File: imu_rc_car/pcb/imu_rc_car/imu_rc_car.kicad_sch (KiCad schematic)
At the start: 27 parts, among them J1 Encoder FS, J10 Prox Sensor RS, J11 Prox Sensor LS, J12 Prox Sensor BS, J2 Encoder BS, J7 Left Terminal, J8 Right Terminal, J9 Prox Sensor FS, Q5 IRLML6344TRPBF, Q6 DMP3160L-7, U1 ESP32-S3-DevKitC, U2 TB6612FNG, U3 AP2112K-3.3, U4 TB6612FNG

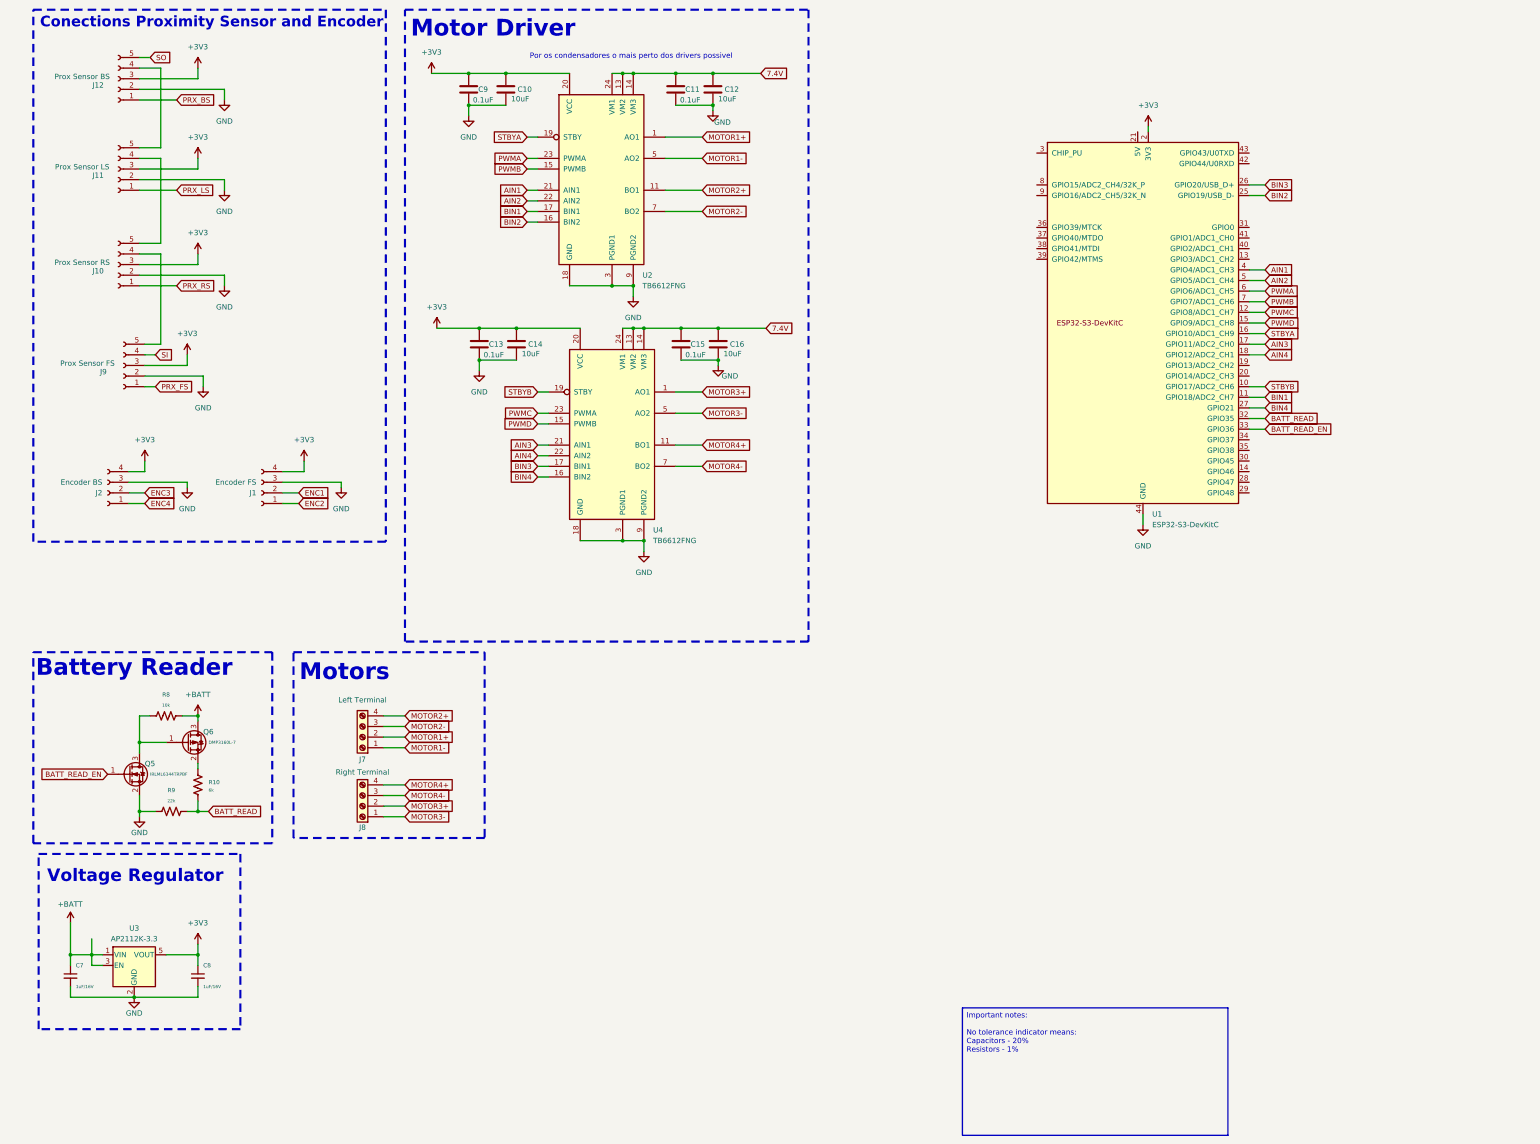
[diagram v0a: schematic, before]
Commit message: commit #27
revision for hand unit complete (board is ready)
board for proximity sensors in series
minor revision in encoder board
progressing work in car board
added essential libraries support for 3D components
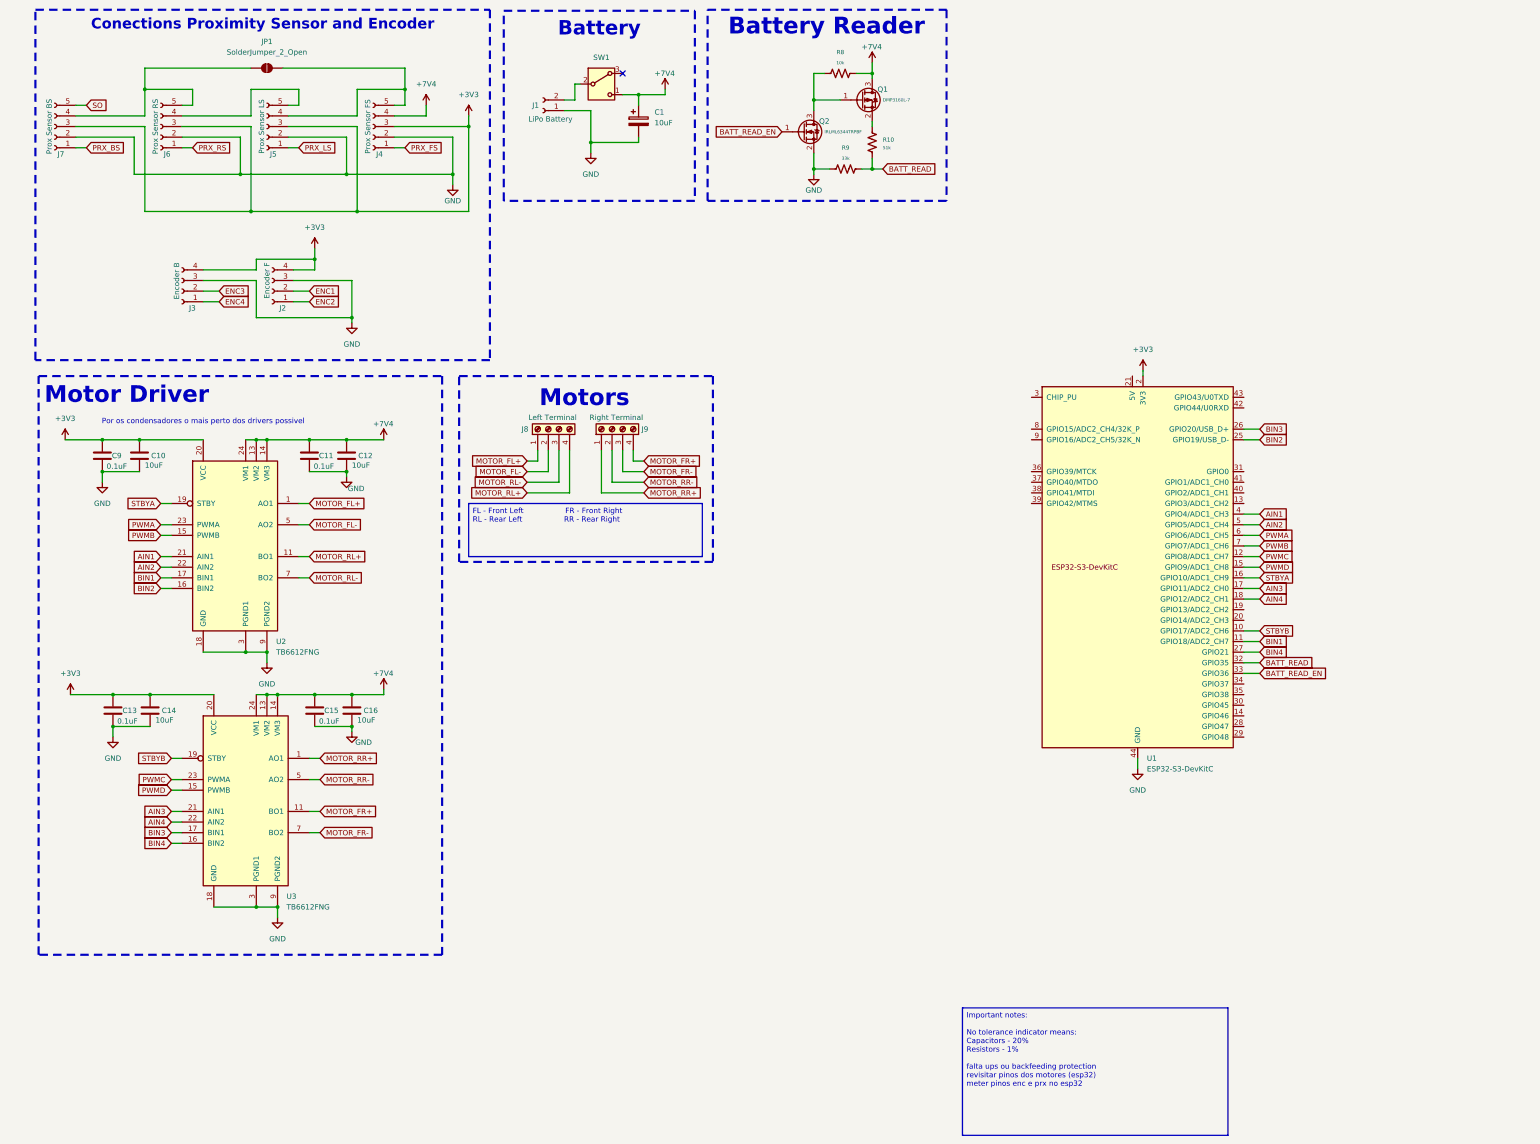
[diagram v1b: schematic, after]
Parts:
- removed C7, C8: 1uF/16V, Capacitor_SMD:C_0805_2012Metric, symbol Device:C_Small
- removed J10: Prox Sensor RS, Connector_JST:JST_PH_S5B-PH-K_1x05_P2.00mm_Horizontal, symbol Connector:Conn_01x05_Socket
- removed J11: Prox Sensor LS, Connector_JST:JST_PH_S5B-PH-K_1x05_P2.00mm_Horizontal, symbol Connector:Conn_01x05_Socket
- removed J12: Prox Sensor BS, Connector_JST:JST_PH_S5B-PH-K_1x05_P2.00mm_Horizontal, symbol Connector:Conn_01x05_Socket
- removed J2: Encoder BS, Connector_JST:JST_PH_S4B-PH-K_1x04_P2.00mm_Horizontal, symbol Connector:Conn_01x04_Socket
- removed U3: AP2112K-3.3, Package_TO_SOT_SMD:SOT-23-5, symbol Regulator_Linear:AP2112K-3.3
- added C1: 10uF, Capacitor_SMD:CP_Elec_5x5.7, symbol Device:C_Polarized
- added J1: LiPo Battery, IMURCLibrary:AMASS_XT60IPW-M_1x03_P7.20mm_Horizontal, symbol Connector:Conn_01x02_Socket
- added J3: Encoder B, IMURCLibrary:JST_PH_S4B-PH-SM4-TB_1x04-1MP_P2.00mm_Horizontal, symbol Connector:Conn_01x04_Socket
- added J5: Prox Sensor LS, IMURCLibrary:JST_PH_S5B-PH-SM4-TB_1x05-1MP_P2.00mm_Horizontal, symbol Connector:Conn_01x05_Socket
- added J6: Prox Sensor RS, IMURCLibrary:JST_PH_S5B-PH-SM4-TB_1x05-1MP_P2.00mm_Horizontal, symbol Connector:Conn_01x05_Socket
- added J7: Prox Sensor BS, IMURCLibrary:JST_PH_S5B-PH-SM4-TB_1x05-1MP_P2.00mm_Horizontal, symbol Connector:Conn_01x05_Socket
- added JP1: SolderJumper_2_Open, Jumper:SolderJumper-2_P1.3mm_Open_RoundedPad1.0x1.5mm, symbol Jumper:SolderJumper_2_Open
- added SW1: SW_Nidec_CAS-120A1, Button_Switch_SMD:Nidec_Copal_CAS-120A, symbol Switch:SW_Nidec_CAS-120A1
- J2: renamed from J1; value Encoder FS -> Encoder F; footprint Connector_JST:JST_PH_S4B-PH-K_1x04_P2.00mm_Horizontal -> IMURCLibrary:JST_PH_S4B-PH-SM4-TB_1x04-1MP_P2.00mm_Horizontal
- J4: renamed from J9; footprint Connector_JST:JST_PH_S5B-PH-K_1x05_P2.00mm_Horizontal -> IMURCLibrary:JST_PH_S5B-PH-SM4-TB_1x05-1MP_P2.00mm_Horizontal
- J8: renamed from J7; footprint TerminalBlock:TerminalBlock_Xinya_XY308-2.54-4P_1x04_P2.54mm_Horizontal -> IMURCLibrary:TerminalBlock_Xinya_XY308-2.54-4P_1x04_P2.54mm_Horizontal
- J9: renamed from J8; footprint TerminalBlock:TerminalBlock_Xinya_XY308-2.54-4P_1x04_P2.54mm_Horizontal -> IMURCLibrary:TerminalBlock_Xinya_XY308-2.54-4P_1x04_P2.54mm_Horizontal
- R10: value 6k -> 51k
- R9: value 22k -> 33k
- U1: footprint PCM_Espressif:ESP32-S3-DevKitC -> IMURCLibrary:ESP32-S3-DevKitC
- renumbered Q6 to Q1, Q5 to Q2, U4 to U3
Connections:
- net 7.4V is gone; now on net +7V4: C11.1, C12.1, C15.1, C16.1, U2.13 (VM2), U2.14 (VM3), U2.24 (VM1), U3.13 (VM2), U3.14 (VM3), U3.24 (VM1)
- net SI is gone; now on net +7V4: J4.4 (Pin_4)
- net +3V3: now also J3.4 (Pin_4), J5.3 (Pin_3), J6.3 (Pin_3), J7.3 (Pin_3)
- net ENC3: now also J3.2 (Pin_2)
- net ENC4: now also J3.1 (Pin_1)
- net GND: now also C1.2, J1.1 (Pin_1), J3.3 (Pin_3), J5.2 (Pin_2), J6.2 (Pin_2), J7.2 (Pin_2)
- net PRX_BS: now also J7.1 (Pin_1)
- net PRX_LS: now also J5.1 (Pin_1)
- net PRX_RS: now also J6.1 (Pin_1)
- net SO: now also J7.5 (Pin_5)
- net at J4.5 (Pin_5): now also J5.4 (Pin_4), JP1.2 (B)
- net +BATT renamed +7V4
- net +7V4: now also C1.1, SW1.1 (C)
- net MOTOR1+ renamed MOTOR_FL+
- net MOTOR_FL+: now also J8.1 (Pin_1); no longer J8.2 (Pin_2)
- net MOTOR1- renamed MOTOR_FL-
- net MOTOR_FL-: now also J8.2 (Pin_2); no longer J8.1 (Pin_1)
- net MOTOR2+ renamed MOTOR_RL+
- net MOTOR2- renamed MOTOR_RL-
- net MOTOR3+ renamed MOTOR_RR+
- net MOTOR_RR+: now also J9.1 (Pin_1); no longer J9.2 (Pin_2)
- net MOTOR3- renamed MOTOR_RR-
- net MOTOR_RR-: now also J9.2 (Pin_2); no longer J9.1 (Pin_1)
- net MOTOR4+ renamed MOTOR_FR+
- net MOTOR4- renamed MOTOR_FR-
- new net: J5.5 (Pin_5), J6.4 (Pin_4)
- new net: J1.2 (Pin_2), SW1.2 (B)
- new net: J6.5 (Pin_5), J7.4 (Pin_4), JP1.1 (A)
- no-connect marks 0 -> 1
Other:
- note added: "Battery"
- note removed: "Voltage Regulator"
- moved on the sheet: C10, C11, C12, C13, C14, C15, C16, C9, J2, J4, J8, J9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

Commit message: commit #28
added 3d file for esp32s3
progression with car pcb
minor changes prox sensors test board
final revision hand unit
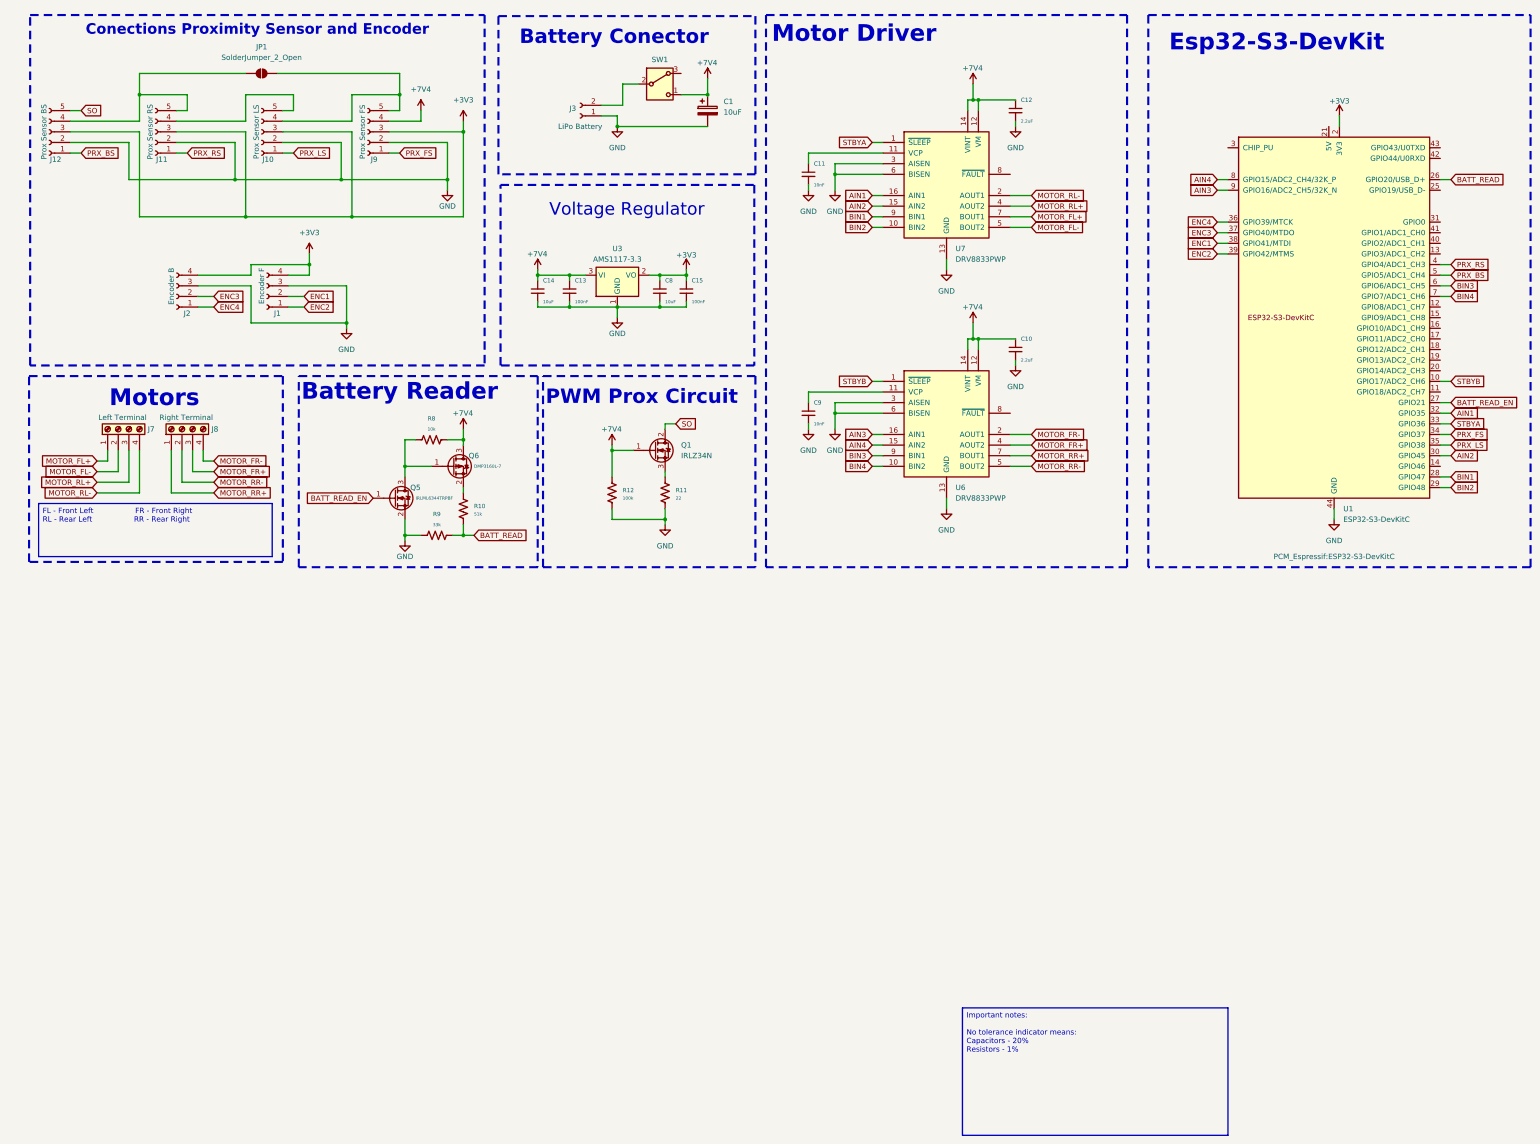
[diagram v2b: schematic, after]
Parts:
- removed C10, C12, C14, C16: 10uF, Capacitor_SMD:C_1206_3216Metric_Pad1.33x1.80mm_HandSolder, symbol Device:C
- removed C11, C13, C15, C9: 0.1uF, Capacitor_SMD:C_1206_3216Metric_Pad1.33x1.80mm_HandSolder, symbol Device:C
- removed U2, U3: TB6612FNG, Package_SO:SSOP-24_5.3x8.2mm_P0.65mm, symbol Driver_Motor:TB6612FNG
- added C10, C12: 2.2uF, Capacitor_SMD:C_0805_2012Metric, symbol Device:C_Small
- added C11, C9: 10nF, Capacitor_SMD:C_0805_2012Metric, symbol Device:C_Small
- added C13, C15: 100nF, Capacitor_SMD:C_0805_2012Metric, symbol Device:C_Small
- added C14, C8: 10uF, Capacitor_SMD:C_0805_2012Metric, symbol Device:C_Small
- added Q1: IRLZ34N, Package_TO_SOT_SMD:TO-263-2_TabPin1, symbol Transistor_FET:IRLZ34N
- added R11: 22, Resistor_SMD:R_0805_2012Metric, symbol Device:R_US
- added R12: 100k, Resistor_SMD:R_0805_2012Metric, symbol Device:R_US
- added U3: AMS1117-3.3, Package_TO_SOT_SMD:SOT-223-3_TabPin2, symbol Regulator_Linear:AMS1117-3.3
- added U6, U7: DRV8833PWP, Package_SO:HTSSOP-16-1EP_4.4x5mm_P0.65mm_EP3.4x5mm_Mask2.46x2.31mm_ThermalVias, symbol Driver_Motor:DRV8833PWP
- J3: renamed from J1; footprint IMURCLibrary:AMASS_XT60IPW-M_1x03_P7.20mm_Horizontal -> TerminalBlock:TerminalBlock_MaiXu_MX126-5.0-02P_1x02_P5.00mm
- SW1: footprint Button_Switch_SMD:Nidec_Copal_CAS-120A -> Button_Switch_THT:SW_Slide_SPDT_Angled_CK_OS102011MA1Q
- U1: footprint IMURCLibrary:ESP32-S3-DevKitC -> PCM_Espressif:ESP32-S3-DevKitC
- renumbered J2 to J1, J5 to J10, J6 to J11, J7 to J12, J3 to J2, J8 to J7, J9 to J8, J4 to J9, Q2 to Q5, Q1 to Q6
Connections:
- net PWMA is gone; now on net BIN3: U1.6 (GPIO6/ADC1_CH5)
- net PWMB is gone; now on net BIN4: U1.7 (GPIO7/ADC1_CH6)
- net +3V3: now also C15.1, C8.1, U3.2 (VO)
- net +7V4: now also C10.1, C12.1, C13.1, C14.1, Q1.1 (G), R12.1, U3.3 (VI), U6.12 (VM), U6.14 (VINT), U7.12 (VM), U7.14 (VINT)
- net AIN1: now also U1.32 (GPIO35), U7.16 (AIN1); no longer U1.4 (GPIO4/ADC1_CH3)
- net AIN2: now also U1.30 (GPIO45), U7.15 (AIN2); no longer U1.5 (GPIO5/ADC1_CH4)
- net AIN3: now also U1.9 (GPIO16/ADC2_CH5/32K_N), U6.16 (AIN1); no longer U1.17 (GPIO11/ADC2_CH0)
- net AIN4: now also U1.8 (GPIO15/ADC2_CH4/32K_P), U6.15 (AIN2); no longer U1.18 (GPIO12/ADC2_CH1)
- net BATT_READ: now also U1.26 (GPIO20/USB_D+); no longer U1.32 (GPIO35)
- net BATT_READ_EN: now also U1.27 (GPIO21); no longer U1.33 (GPIO36)
- net BIN1: now also U1.28 (GPIO47), U7.9 (BIN1); no longer U1.11 (GPIO18/ADC2_CH7)
- net BIN2: now also U1.29 (GPIO48), U7.10 (BIN2); no longer U1.25 (GPIO19/USB_D-)
- net BIN3: now also U6.9 (BIN1); no longer U1.26 (GPIO20/USB_D+)
- net BIN4: now also U6.10 (BIN2); no longer U1.27 (GPIO21)
- net ENC1: now also U1.38 (GPIO41/MTDI)
- net ENC2: now also U1.39 (GPIO42/MTMS)
- net ENC3: now also U1.37 (GPIO40/MTDO)
- net ENC4: now also U1.36 (GPIO39/MTCK)
- net GND: now also C10.2, C11.2, C12.2, C13.2, C14.2, C15.2, C8.2, C9.2, R11.2, R12.2, U3.1 (GND), U6.13 (GND), U6.17 (GND), U6.3 (AISEN), U6.6 (BISEN), U7.13 (GND), U7.17 (GND), U7.3 (AISEN), U7.6 (BISEN)
- net MOTOR_FL+: now also U7.7 (BOUT1)
- net MOTOR_FL-: now also U7.5 (BOUT2)
- net MOTOR_FR+: now also J8.3 (Pin_3), U6.4 (AOUT2); no longer J8.4 (Pin_4)
- net MOTOR_FR-: now also J8.4 (Pin_4), U6.2 (AOUT1); no longer J8.3 (Pin_3)
- net MOTOR_RL+: now also J7.3 (Pin_3), U7.4 (AOUT2); no longer J7.4 (Pin_4)
- net MOTOR_RL-: now also J7.4 (Pin_4), U7.2 (AOUT1); no longer J7.3 (Pin_3)
- net MOTOR_RR+: now also U6.7 (BOUT1)
- net MOTOR_RR-: now also U6.5 (BOUT2)
- net PRX_BS: now also U1.5 (GPIO5/ADC1_CH4)
- net PRX_FS: now also U1.34 (GPIO37)
- net PRX_LS: now also U1.35 (GPIO38)
- net PRX_RS: now also U1.4 (GPIO4/ADC1_CH3)
- net SO: now also Q1.2 (D)
- net STBYA: now also U1.33 (GPIO36), U7.1 (~{SLEEP}); no longer U1.16 (GPIO10/ADC1_CH9)
- net STBYB: now also U6.1 (~{SLEEP})
- net PWMC: no longer names the net of U1.12 (GPIO8/ADC1_CH7)
- net PWMD: no longer names the net of U1.15 (GPIO9/ADC1_CH8)
- new net: C11.1, U7.11 (VCP)
- new net: C9.1, U6.11 (VCP)
- new net: Q1.3 (S), R11.1
- no-connect marks 1 -> 0
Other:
- note added: "Battery Conector"
- note added: "Esp32-S3-DevKit"
- note added: "PWM Prox Circuit"
- note added: "Voltage Regulator"
- note removed: "Battery"
- note removed: "Por os condensadores o mais perto dos drivers possivel"
- moved on the sheet: J1, J10, J11, J12, J2, J3, J7, J8, J9, JP1, Q5, Q6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
